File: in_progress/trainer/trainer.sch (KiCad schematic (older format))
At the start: 55 parts, among them CON1 BARREL_JACK, P1 CONN_01X02, P11 CONN_01X03, P2 CONN_02X02, P3 CONN_01X04, P4 CONN_02X08, P5 USB_A, Q1 2N3904, Q2 2N3904, U1 LM7805, U2 LM3940, U3 ULN2803A, U4 ULN2803A, X1 Buzzer_Son

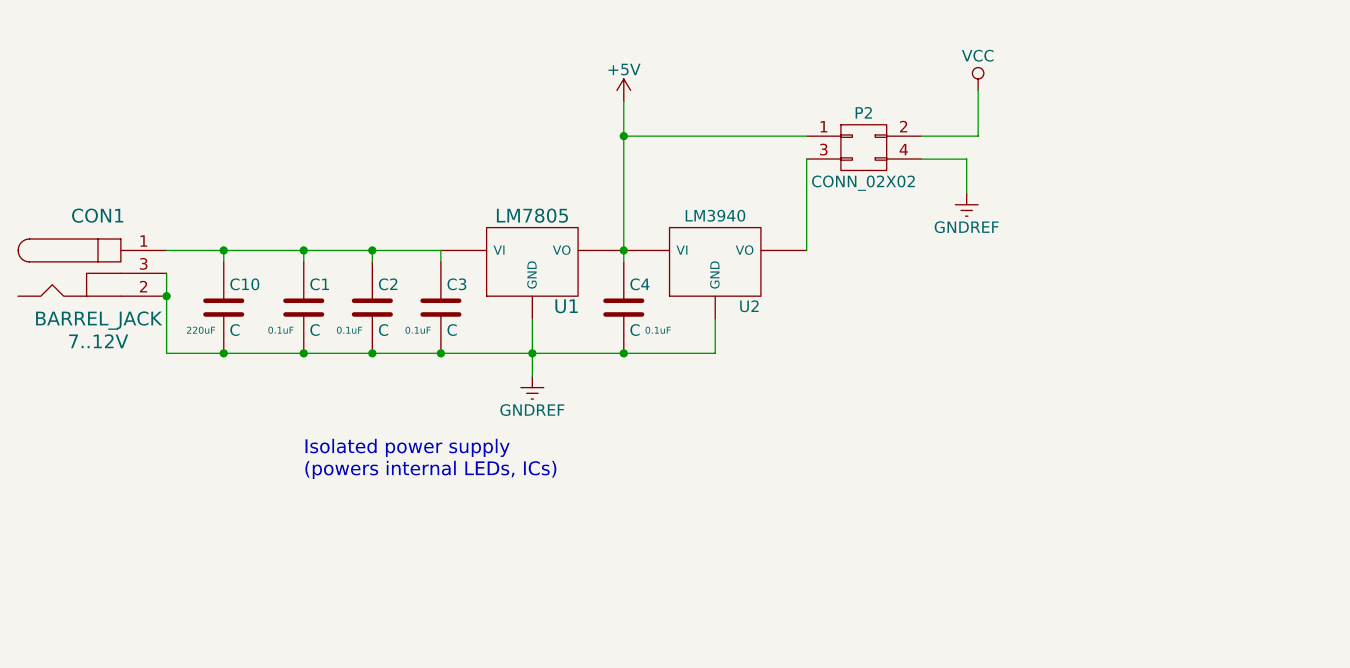
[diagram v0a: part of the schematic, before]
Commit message: .
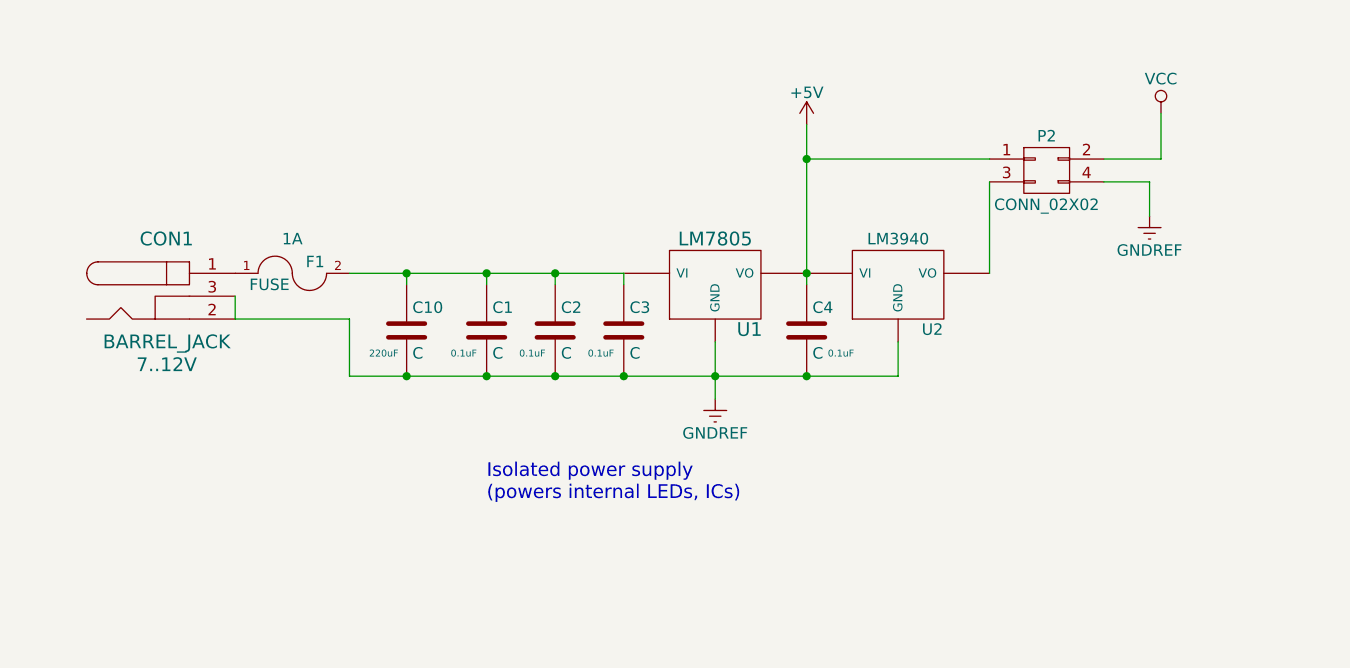
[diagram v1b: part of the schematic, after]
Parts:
- added F1: FUSE, 1A, symbol FUSE
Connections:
- net at C1.1, C10.1, C2.1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: now also F1.2; no longer CON1.1
- new net: CON1.1, F1.1
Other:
- moved on the sheet: C1, C10, C2, C3, C4, CON1, P2, U1, U2
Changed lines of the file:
@@
 L C-RESCUE-trainer C3
 U 1 1 5657DDA5
-P 2900 2050
-F 0 "C3" H 2925 2150 50  0000 L CNN
-F 1 "C" H 2925 1950 50  0000 L CNN
-F 2 "0.1uF" H 2800 1950 30  0000 C CNN
-F 3 "" H 2900 2050 60  0000 C CNN
-	1    2900 2050
+P 3700 2150
+F 0 "C3" H 3725 2250 50  0000 L CNN
+F 1 "C" H 3725 2050 50  0000 L CNN
+F 2 "0.1uF" H 3600 2050 30  0000 C CNN
+F 3 "" H 3700 2150 60  0000 C CNN
+	1    3700 2150
 	1    0    0    -1
 $EndComp
@@
 L C-RESCUE-trainer C4
 U 1 1 5657DE9C
-P 3700 2050
-F 0 "C4" H 3725 2150 50  0000 L CNN
-F 1 "C" H 3725 1950 50  0000 L CNN
-F 2 "0.1uF" H 3850 1950 30  0000 C CNN
-F 3 "" H 3700 2050 60  0000 C CNN
-	1    3700 2050
+P 4500 2150
+F 0 "C4" H 4525 2250 50  0000 L CNN
+F 1 "C" H 4525 2050 50  0000 L CNN
+F 2 "0.1uF" H 4650 2050 30  0000 C CNN
+F 3 "" H 4500 2150 60  0000 C CNN
+	1    4500 2150
 	1    0    0    -1
 $EndComp
@@
 L GNDREF #PWR5
 U 1 1 5657E02B
-P 3300 2350
-F 0 "#PWR5" H 3300 2100 50  0001 C CNN
-F 1 "GNDREF" H 3300 2200 50  0000 C CNN
-F 2 "" H 3300 2350 60  0000 C CNN
-F 3 "" H 3300 2350 60  0000 C CNN
-	1    3300 2350
+P 4100 2450
+F 0 "#PWR5" H 4100 2200 50  0001 C CNN
+F 1 "GNDREF" H 4100 2300 50  0000 C CNN
+F 2 "" H 4100 2450 60  0000 C CNN
+F 3 "" H 4100 2450 60  0000 C CNN
+	1    4100 2450
 	1    0    0    -1
 $EndComp
@@
 L +5V #PWR6
 U 1 1 5657E06F
-P 3700 1150
-F 0 "#PWR6" H 3700 1000 50  0001 C CNN
-F 1 "+5V" H 3700 1290 50  0000 C CNN
-F 2 "" H 3700 1150 60  0000 C CNN
-F 3 "" H 3700 1150 60  0000 C CNN
-	1    3700 1150
+P 4500 1250
+F 0 "#PWR6" H 4500 1100 50  0001 C CNN
+F 1 "+5V" H 4500 1390 50  0000 C CNN
+F 2 "" H 4500 1250 60  0000 C CNN
+F 3 "" H 4500 1250 60  0000 C CNN
+	1    4500 1250
 	1    0    0    -1
 $EndComp
@@
 L BARREL_JACK CON1
 U 1 1 56587C69
-P 1400 1900
-F 0 "CON1" H 1400 2150 60  0000 C CNN
-F 1 "BARREL_JACK" H 1400 1700 60  0000 C CNN
-F 2 "7..12V" H 1400 1600 60  0000 C CNN
-F 3 "" H 1400 1900 60  0000 C CNN
-	1    1400 1900
+P 1700 2000
+F 0 "CON1" H 1700 2250 60  0000 C CNN
+F 1 "BARREL_JACK" H 1700 1800 60  0000 C CNN
+F 2 "7..12V" H 1700 1700 60  0000 C CNN
+F 3 "" H 1700 2000 60  0000 C CNN
+	1    1700 2000
 	1    0    0    -1
 $EndComp
@@
 L VCC #PWR8
 U 1 1 565A8B1D
-P 5250 1100
-F 0 "#PWR8" H 5250 950 50  0001 C CNN
-F 1 "VCC" H 5250 1250 50  0000 C CNN
-F 2 "" H 5250 1100 60  0000 C CNN
-F 3 "" H 5250 1100 60  0000 C CNN
-	1    5250 1100
+P 6050 1200
+F 0 "#PWR8" H 6050 1050 50  0001 C CNN
+F 1 "VCC" H 6050 1350 50  0000 C CNN
+F 2 "" H 6050 1200 60  0000 C CNN
+F 3 "" H 6050 1200 60  0000 C CNN
+	1    6050 1200
 	1    0    0    -1
 $EndComp
@@
 L GNDREF #PWR7
 U 1 1 565A8FBD
-P 5200 1550
-F 0 "#PWR7" H 5200 1300 50  0001 C CNN
-F 1 "GNDREF" H 5200 1400 50  0000 C CNN
-F 2 "" H 5200 1550 60  0000 C CNN
-F 3 "" H 5200 1550 60  0000 C CNN
-	1    5200 1550
-	1    0    0    -1
-$EndComp
-Text Notes 2300 2800 0    60   ~ 0
+P 6000 1650
+F 0 "#PWR7" H 6000 1400 50  0001 C CNN
+F 1 "GNDREF" H 6000 1500 50  0000 C CNN
+F 2 "" H 6000 1650 60  0000 C CNN
+F 3 "" H 6000 1650 60  0000 C CNN
+	1    6000 1650
+	1    0    0    -1
+$EndComp
+Text Notes 3100 2900 0    60   ~ 0
 Isolated power supply\n(powers internal LEDs, ICs)
 $Sheet
@@
 L C-RESCUE-trainer C2
 U 1 1 568F03CD
-P 2600 2050
-F 0 "C2" H 2625 2150 50  0000 L CNN
-F 1 "C" H 2625 1950 50  0000 L CNN
-F 2 "0.1uF" H 2500 1950 30  0000 C CNN
-F 3 "" H 2600 2050 60  0000 C CNN
-	1    2600 2050
+P 3400 2150
+F 0 "C2" H 3425 2250 50  0000 L CNN
+F 1 "C" H 3425 2050 50  0000 L CNN
+F 2 "0.1uF" H 3300 2050 30  0000 C CNN
+F 3 "" H 3400 2150 60  0000 C CNN
+	1    3400 2150
 	1    0    0    -1
 $EndComp
@@
 L C-RESCUE-trainer C1
 U 1 1 568F048E
-P 2300 2050
-F 0 "C1" H 2325 2150 50  0000 L CNN
-F 1 "C" H 2325 1950 50  0000 L CNN
-F 2 "0.1uF" H 2200 1950 30  0000 C CNN
-F 3 "" H 2300 2050 60  0000 C CNN
-	1    2300 2050
+P 3100 2150
+F 0 "C1" H 3125 2250 50  0000 L CNN
+F 1 "C" H 3125 2050 50  0000 L CNN
+F 2 "0.1uF" H 3000 2050 30  0000 C CNN
+F 3 "" H 3100 2150 60  0000 C CNN
+	1    3100 2150
 	1    0    0    -1
 $EndComp
@@
 L LM7805 U1
 U 1 1 5657C7C3
-P 3300 1850
-F 0 "U1" H 3450 1654 60  0000 C CNN
-F 1 "LM7805" H 3300 2050 60  0000 C CNN
-F 2 "" H 3300 1850 60  0000 C CNN
-F 3 "" H 3300 1850 60  0000 C CNN
-	1    3300 1850
+P 4100 1950
+F 0 "U1" H 4250 1754 60  0000 C CNN
+F 1 "LM7805" H 4100 2150 60  0000 C CNN
+F 2 "" H 4100 1950 60  0000 C CNN
+F 3 "" H 4100 1950 60  0000 C CNN
+	1    4100 1950
 	1    0    0    -1
 $EndComp
@@
 	7900 2150 7900 1500
 Wire Wire Line
-	1700 1800 2900 1800
-Wire Wire Line
-	3700 1150 3700 1850
-Wire Wire Line
-	1700 1900 1700 2250
-Connection ~ 1700 2000
-Wire Wire Line
-	3300 2100 3300 2350
-Connection ~ 3300 2250
+	2500 1900 3700 1900
+Wire Wire Line
+	4500 1250 4500 1950
+Wire Wire Line
+	4100 2200 4100 2450
+Connection ~ 4100 2350
 Wire Wire Line
 	7700 1800 7300 1800
@@
 Wire Wire Line
 	7600 1700 7600 1500
-Connection ~ 3700 1800
+Connection ~ 4500 1900
 Wire Wire Line
 	1550 6900 2050 6900
@@
 Connection ~ 2800 4000
 Wire Wire Line
-	2300 1850 2300 1800
-Connection ~ 2300 1800
-Wire Wire Line
-	2600 1850 2600 1800
-Connection ~ 2600 1800
-Wire Wire Line
-	2900 1800 2900 1850
+	3100 1950 3100 1900
+Connection ~ 3100 1900
+Wire Wire Line
+	3400 1950 3400 1900
+Connection ~ 3400 1900
+Wire Wire Line
+	3700 1900 3700 1950
 $Comp
 L CONN_01X02 P1
@@
 L CONN_02X02 P2
 U 1 1 566EE3C5
-P 4750 1350
-F 0 "P2" H 4750 1500 50  0000 C CNN
-F 1 "CONN_02X02" H 4750 1200 50  0000 C CNN
-F 2 "" H 4750 150 50  0000 C CNN
-F 3 "" H 4750 150 50  0000 C CNN
-	1    4750 1350
+P 5550 1450
+F 0 "P2" H 5550 1600 50  0000 C CNN
+F 1 "CONN_02X02" H 5550 1300 50  0000 C CNN
+F 2 "" H 5550 250 50  0000 C CNN
+F 3 "" H 5550 250 50  0000 C CNN
+	1    5550 1450
 	1    0    0    -1
 $EndComp
@@
 L LM7805 U2
 U 1 1 566EF639
-P 4100 1850
-F 0 "U2" H 4250 1654 50  0000 C CNN
-F 1 "LM3940" H 4100 2050 50  0000 C CNN
-F 2 "" H 4100 1850 50  0000 C CNN
-F 3 "" H 4100 1850 50  0000 C CNN
-	1    4100 1850
-	1    0    0    -1
-$EndComp
-Wire Wire Line
-	4500 1400 4500 1800
-Wire Wire Line
-	4500 1300 3700 1300
-Connection ~ 3700 1300
-Wire Wire Line
-	5000 1300 5250 1300
-Wire Wire Line
-	5250 1300 5250 1100
-Wire Wire Line
-	5000 1400 5200 1400
-Wire Wire Line
-	5200 1400 5200 1550
-Wire Wire Line
-	4100 2250 4100 2100
-Connection ~ 3700 2250
+P 4900 1950
+F 0 "U2" H 5050 1754 50  0000 C CNN
+F 1 "LM3940" H 4900 2150 50  0000 C CNN
+F 2 "" H 4900 1950 50  0000 C CNN
+F 3 "" H 4900 1950 50  0000 C CNN
+	1    4900 1950
+	1    0    0    -1
+$EndComp
+Wire Wire Line
+	5300 1500 5300 1900
+Wire Wire Line
+	5300 1400 4500 1400
+Connection ~ 4500 1400
+Wire Wire Line
+	5800 1400 6050 1400
+Wire Wire Line
+	6050 1400 6050 1200
+Wire Wire Line
+	5800 1500 6000 1500
+Wire Wire Line
+	6000 1500 6000 1650
+Wire Wire Line
+	4900 2350 4900 2200
+Connection ~ 4500 2350
 NoConn ~ 8950 4450
 NoConn ~ 8950 5700
-Connection ~ 2300 2250
-Connection ~ 2600 2250
-Connection ~ 2900 2250
+Connection ~ 3100 2350
+Connection ~ 3400 2350
+Connection ~ 3700 2350
 $Comp
 L CONN_01X04 P3
@@
 L C-RESCUE-trainer C10
 U 1 1 5671B0F2
-P 1950 2050
-F 0 "C10" H 1975 2150 50  0000 L CNN
-F 1 "C" H 1975 1950 50  0000 L CNN
-F 2 "220uF" H 1850 1950 30  0000 C CNN
-F 3 "" H 1950 2050 60  0000 C CNN
-	1    1950 2050
-	1    0    0    -1
-$EndComp
-Wire Wire Line
-	1700 2250 4100 2250
-Connection ~ 1950 2250
-Wire Wire Line
-	1950 1850 1950 1800
-Connection ~ 1950 1800
+P 2750 2150
+F 0 "C10" H 2775 2250 50  0000 L CNN
+F 1 "C" H 2775 2050 50  0000 L CNN
+F 2 "220uF" H 2650 2050 30  0000 C CNN
+F 3 "" H 2750 2150 60  0000 C CNN
+	1    2750 2150
+	1    0    0    -1
+$EndComp
+Wire Wire Line
+	2500 2350 4900 2350
+Connection ~ 2750 2350
+Wire Wire Line
+	2750 1950 2750 1900
+Connection ~ 2750 1900
+$Comp
+L FUSE F1
+U 1 1 566F2822
+P 2250 1900
+F 0 "F1" H 2350 1950 50  0000 C CNN
+F 1 "FUSE" H 2150 1850 50  0000 C CNN
+F 2 "1A" H 2250 2050 50  0000 C CNN
+F 3 "" H 2250 1900 50  0000 C CNN
+	1    2250 1900
+	1    0    0    -1
+$EndComp
+Wire Wire Line
+	2000 2000 2000 2100
+Wire Wire Line
+	2000 2100 2500 2100
+Wire Wire Line
+	2500 2100 2500 2350
 $EndSCHEMATC

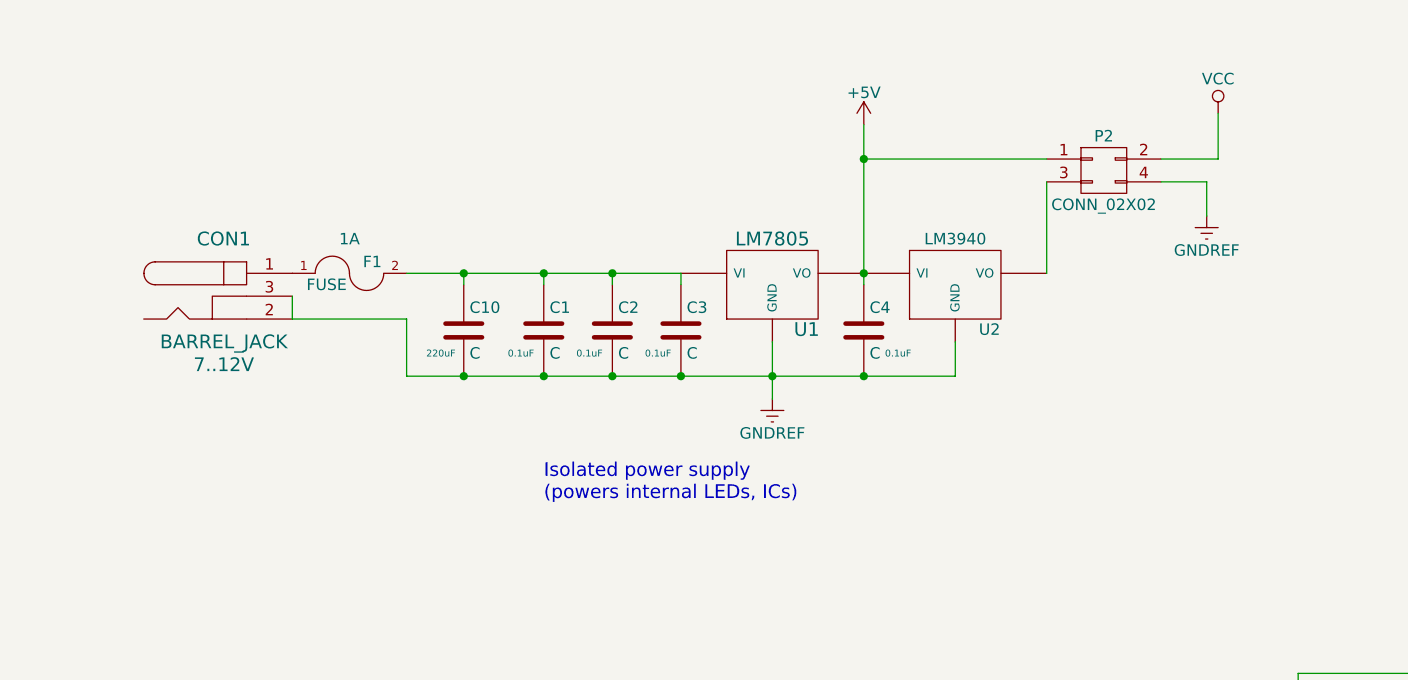
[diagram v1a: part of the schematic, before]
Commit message: .
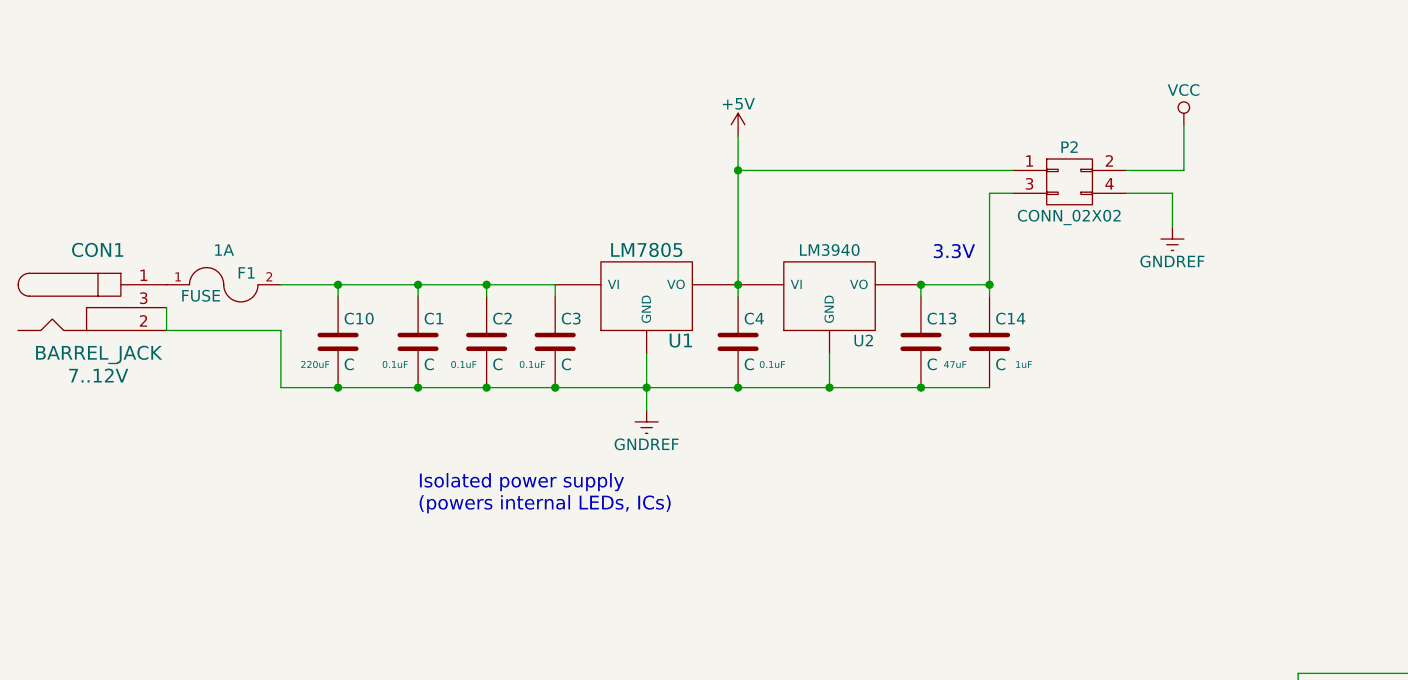
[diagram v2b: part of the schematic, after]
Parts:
- added C13: C, 47uF, symbol C-RESCUE-trainer
- added C14: C, 1uF, symbol C-RESCUE-trainer
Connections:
- net GNDREF: now also C13.2, C14.2
- net at P2.3 (P3), U2.VO: now also C13.1, C14.1
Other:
- note added: "3.3V"
- moved on the sheet: C1, C10, C2, C3, C4, CON1, F1, P2, U1, U2
